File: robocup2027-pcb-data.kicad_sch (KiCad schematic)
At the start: 46 parts, among them M5 Motor_Servo, M6 Motor_Servo, Q1 BPW40, Q2 BPW40, U1 ESP32-DEVKITC-32E

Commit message: assigned footprints and added them to pcb
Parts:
- U13: footprint (none) -> robo:fe-urt-2
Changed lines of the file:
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@@
 			)
 		)
-		(property "Footprint" ""
+		(property "Footprint" "robo:fe-urt-2"
 			(at 314.96 35.56 0)
 			(effects

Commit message: update
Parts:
- S1, S2: footprint robo:DS-850K-S-ON -> robo:CW-SB11KKFF
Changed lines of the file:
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@@
 			)
 		)
-		(property "Footprint" "robo:DS-850K-S-ON"
+		(property "Footprint" "robo:CW-SB11KKFF"
 			(at 86.36 133.35 0)
 			(effects
@@
 			)
 		)
-		(property "Footprint" "robo:DS-850K-S-ON"
+		(property "Footprint" "robo:CW-SB11KKFF"
 			(at 38.1 38.1 0)
 			(effects

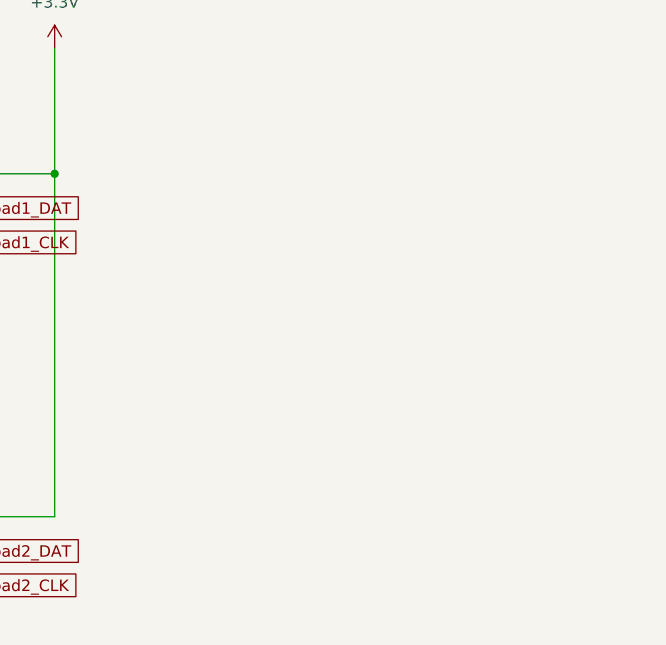
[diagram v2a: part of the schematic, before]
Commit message: placing bno550
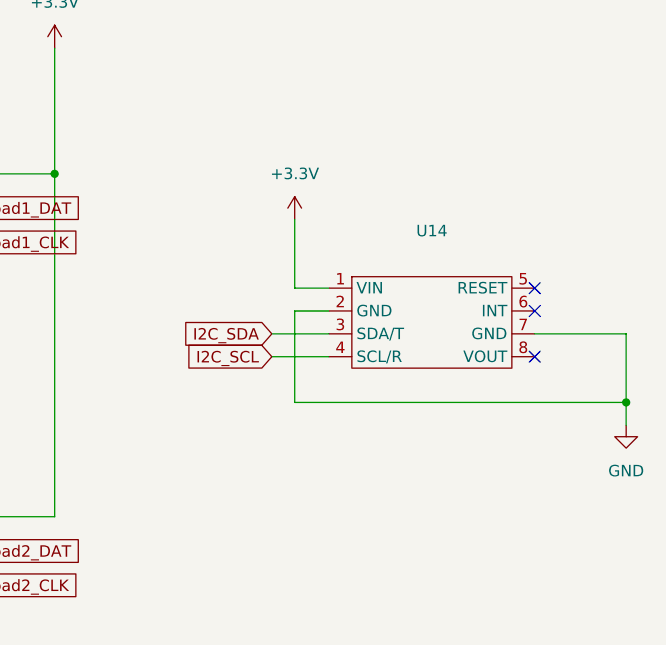
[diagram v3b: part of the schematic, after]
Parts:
- added U14: ~, robo:AE-BNO055-BO, symbol robo:AE-BNO055-BO
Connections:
- net +3.3V: now also U14.1 (VIN)
- net GND: now also U14.2 (GND), U14.7 (GND)
- net I2C_SCL: now also U14.4 (SCL/R)
- net I2C_SDA: now also U14.3 (SDA/T)
- no-connect marks 49 -> 52

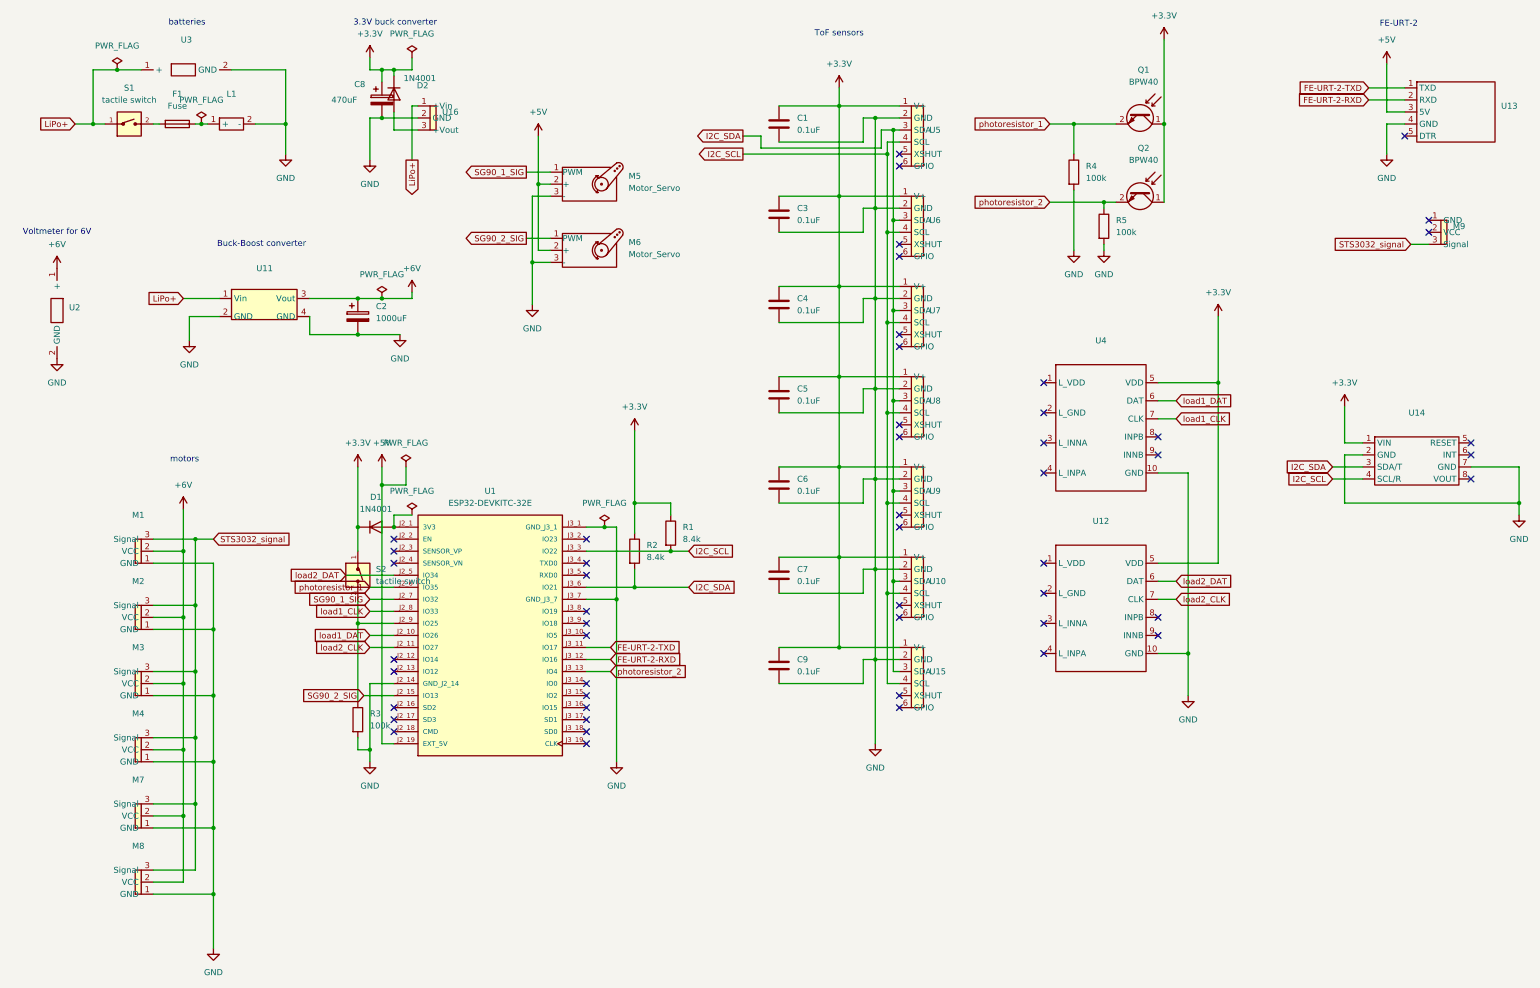
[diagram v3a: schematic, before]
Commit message: update
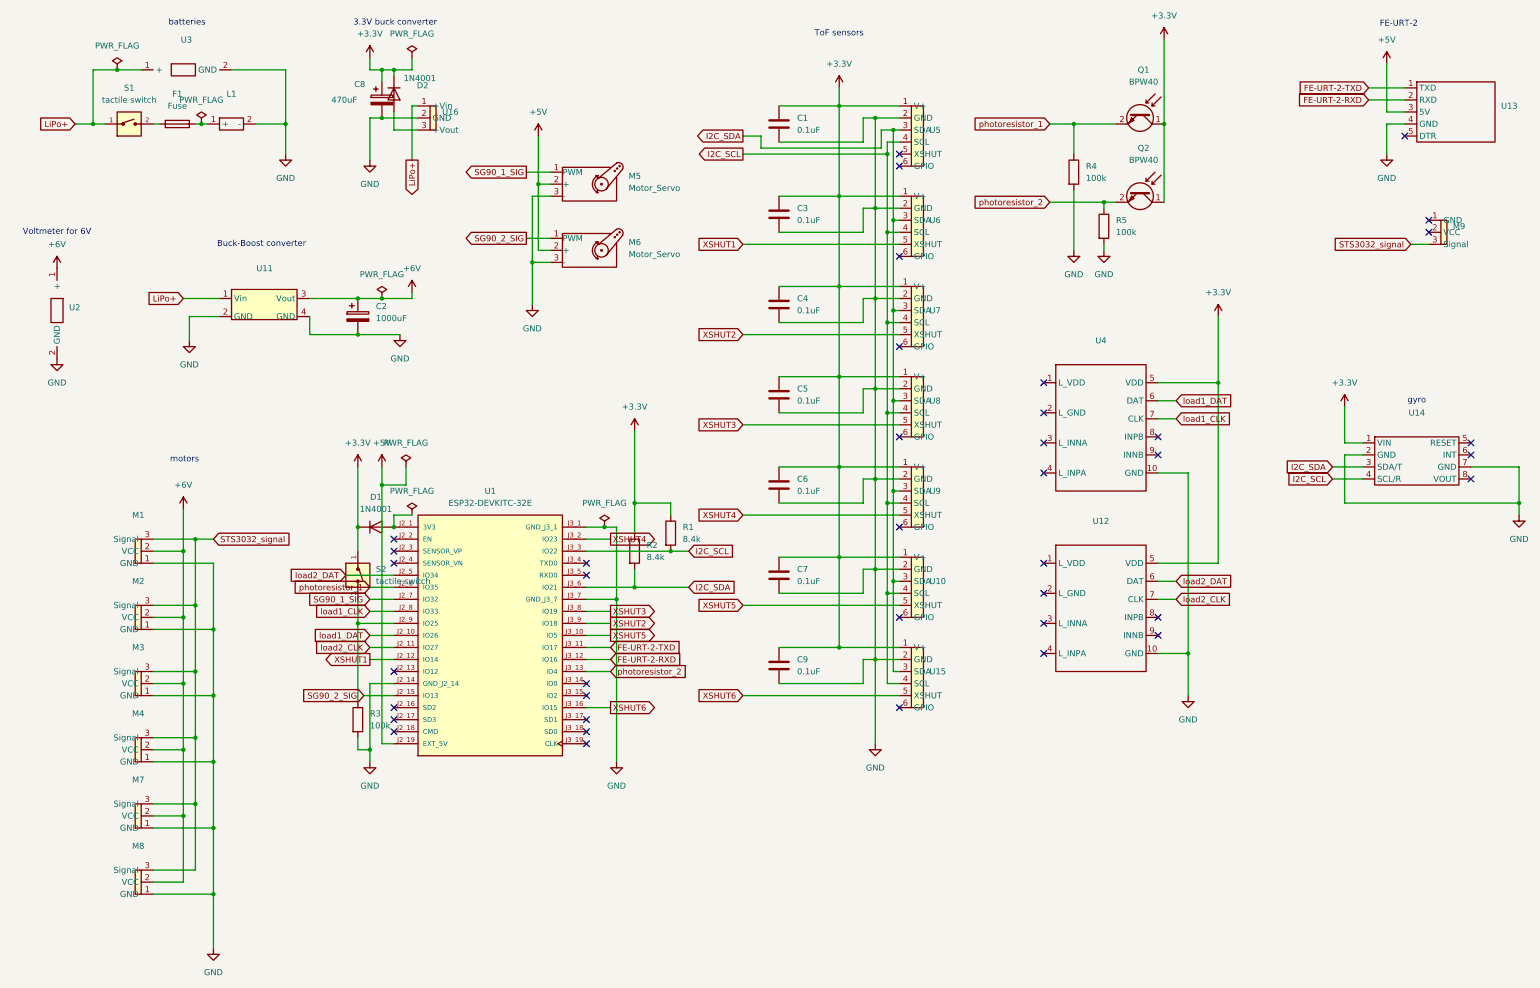
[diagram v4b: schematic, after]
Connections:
- net XSHUT2: now reaches U7.5 (XSHUT)
- net XSHUT2: now also U1.J3_9 (IO18)
- net XSHUT1: now reaches U1.J2_12 (IO14)
- net XSHUT1: now also U6.5 (XSHUT)
- net XSHUT5: now reaches U1.J3_10 (IO5)
- net XSHUT5: now also U10.5 (XSHUT)
- net XSHUT6: now reaches U1.J3_16 (IO15)
- net XSHUT6: now also U15.5 (XSHUT)
- net XSHUT4: now reaches U1.J3_2 (IO23)
- net XSHUT4: now also U9.5 (XSHUT)
- net XSHUT3: now reaches U1.J3_8 (IO19)
- net XSHUT3: now also U8.5 (XSHUT)
- no-connect marks 52 -> 40
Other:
- note added: "gyro"
